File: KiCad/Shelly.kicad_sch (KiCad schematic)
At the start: 26 parts, among them J1 Shelly 1, J2 Other, J3 USB-C, Q1 PMF170XP,115, Q2 PMF250XNEX, U1 FT231XQ, U2 LMR16006X

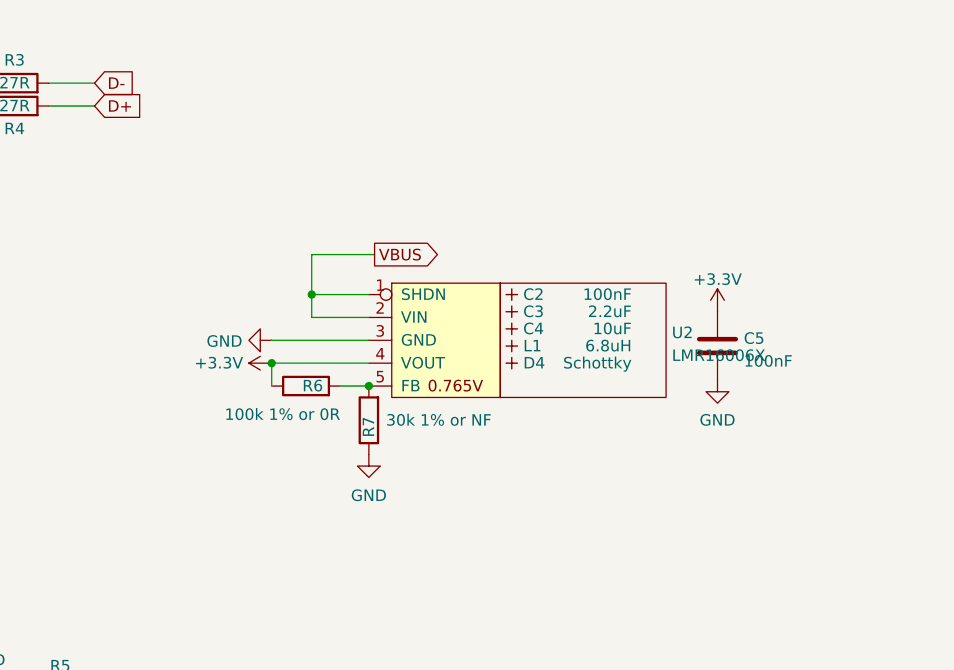
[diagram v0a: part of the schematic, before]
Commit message: Production order
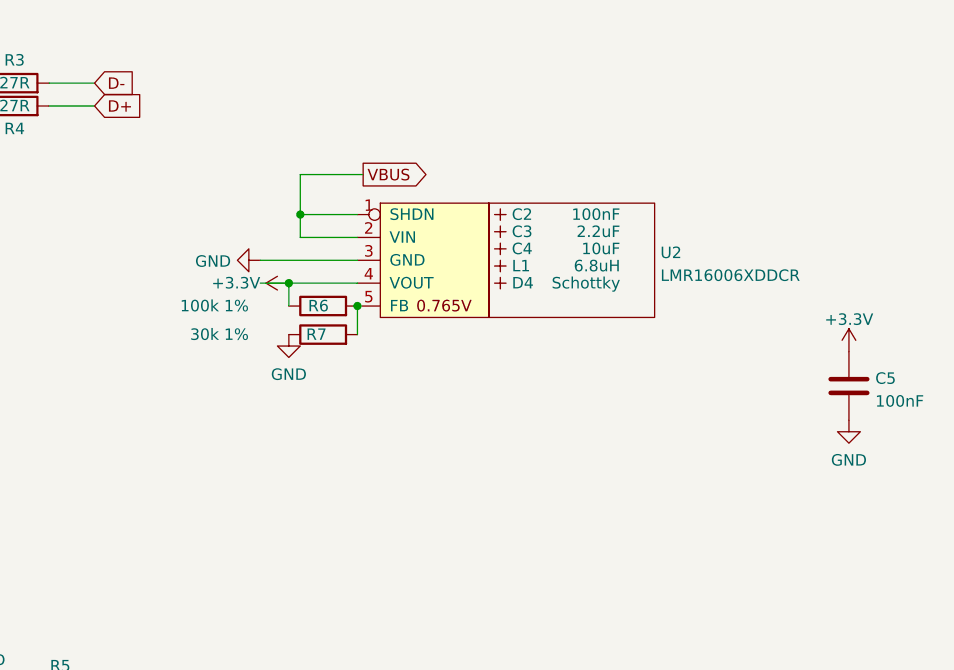
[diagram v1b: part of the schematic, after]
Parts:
- C2: LCSC Part # (none) -> C30926
- C3: LCSC Part # (none) -> C19110
- C4: LCSC Part # (none) -> C17024
- D1, D2: footprint Package_TO_SOT_SMD:SOT-363_SC-70-6 -> RevK:SOT-363_SC-70-6-Rot; LCSC Part # (none) -> C68987
- D3: LCSC Part # (none) -> C264473
- D4: LCSC Part # (none) -> C143805; Part No CD1206-B2100 -> (none)
- J1: footprint Connector_PinHeader_2.54mm:PinHeader_1x05_P2.54mm_Vertical -> RevK:PinHeader_1x05_P2.54mm_Right; LCSC Part # (none) -> C225491; now in the parts list
- J2: footprint Connector_PinHeader_1.27mm:PinHeader_1x06_P1.27mm_Vertical -> RevK:PinHeader_1x06_P1.27mm_Vertical; LCSC Part # (none) -> C2832273; now in the parts list
- J3: LCSC Part # (none) -> C709357; Note Available from Toby Electronics -> (none)
- L1: footprint RevK:L_4x4_ -> RevK:L_1210_; LCSC Part # (none) -> C560045; Manufacturer Laird -> (none); Part No TYA4020 -> (none)
- Q1, Q2: footprint Package_TO_SOT_SMD:SOT-323_SC-70 -> RevK:SOT-323_SC-70
- R6: value 100k 1% or 0R -> 100k 1%; LCSC Part # (none) -> C14675
- R7: value 30k 1% or NF -> 30k 1%; LCSC Part # (none) -> C100001
- U1: footprint RevK:QFN-20-1EP_4x4mm_P0.5mm_EP2.5x2.5mm -> RevK:QFN-20-1EP_4x4mm_P0.5mm_EP2.5x2.5mm-Rot; LCSC Part # (none) -> C132159
- U2: value LMR16006X -> LMR16006XDDCR; footprint RevK:SOT-23-Thin-6-Reg -> RevK:SOT-23-Thin-6-Reg2; LCSC Part # (none) -> C87080; Manufacturer TI -> (none); Part No LMR16006X -> (none)
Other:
- moved on the sheet: C5
